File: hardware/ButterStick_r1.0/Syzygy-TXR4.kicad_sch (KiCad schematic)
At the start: 19 parts, among them J5 SYZYGY-TXR-4, U15 TLV62569DRL

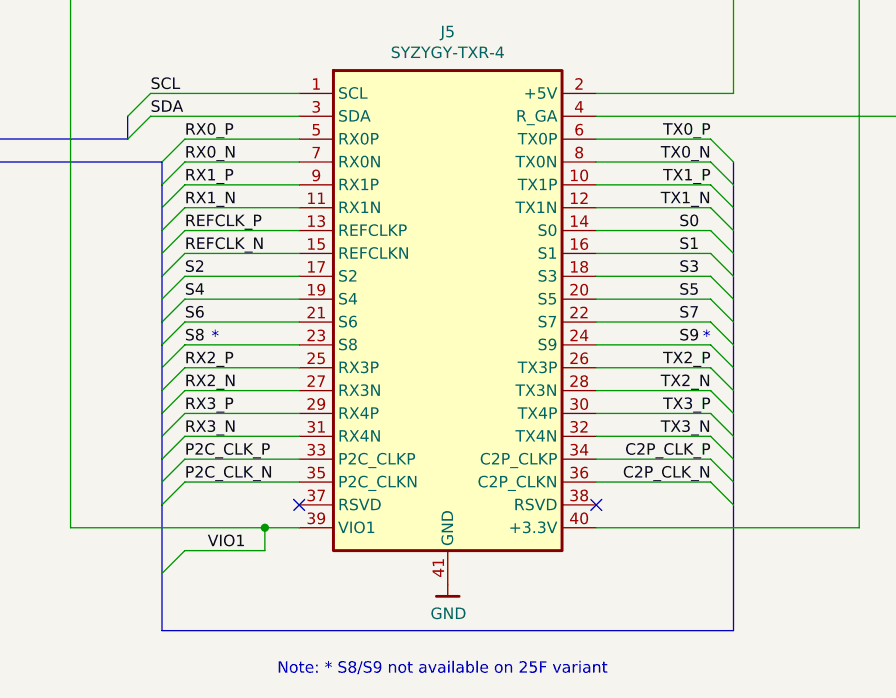
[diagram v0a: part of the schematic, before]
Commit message: hw.r1d0: Review complete, gerbers generated
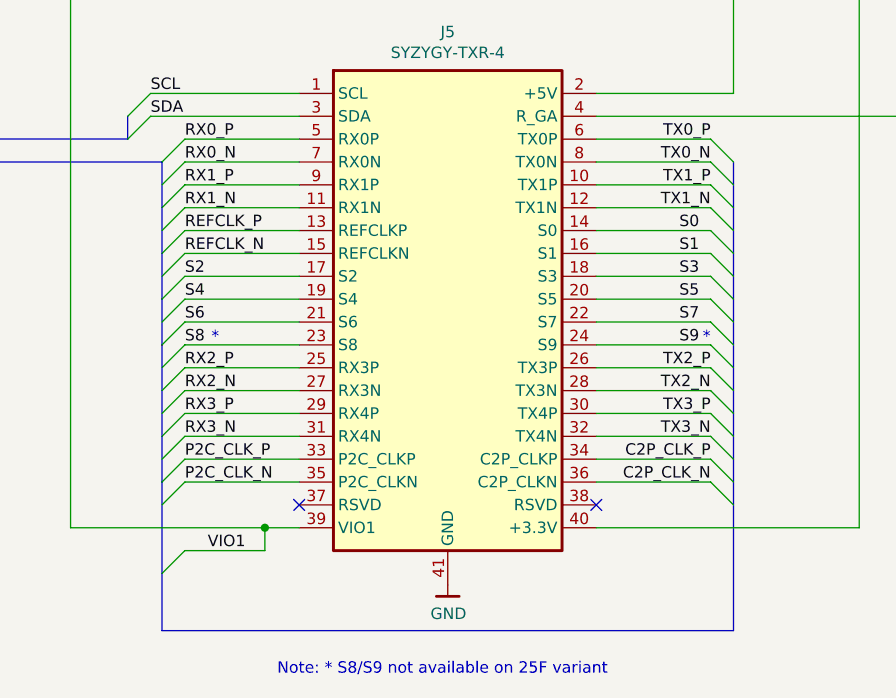
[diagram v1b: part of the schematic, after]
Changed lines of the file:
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@@
   (title_block
     (title "ButterStick")
-    (date "2020-07-16")
+    (date "2020-07-17")
     (rev "r1.0")
     (company "GsD")
@@
   (junction (at 137.16 39.37) (diameter 0) (color 0 0 0 0))
   (junction (at 176.53 142.24) (diameter 0) (color 0 0 0 0))
+  (no_connect (at 180.34 139.7))
   (no_connect (at 213.36 139.7))
-  (no_connect (at 180.34 139.7))
   (bus_entry (at 161.29 96.52) (size 2.54 -2.54)
     (stroke (width 0.1524) (type solid) (color 0 0 0 0))
@@
     (stroke (width 0) (type solid) (color 0 0 0 0))
   )
-  (bus (pts (xy 165.1 101.6) (xy 165.1 104.14))
-    (stroke (width 0) (type solid) (color 0 0 0 0))
-  )
-  (bus (pts (xy 165.1 104.14) (xy 165.1 109.22))
-    (stroke (width 0) (type solid) (color 0 0 0 0))
-  )
-  (bus (pts (xy 165.1 109.22) (xy 165.1 114.3))
-    (stroke (width 0) (type solid) (color 0 0 0 0))
-  )
-  (bus (pts (xy 165.1 114.3) (xy 165.1 119.38))
-    (stroke (width 0) (type solid) (color 0 0 0 0))
-  )
-  (bus (pts (xy 165.1 119.38) (xy 165.1 121.92))
+  (bus (pts (xy 165.1 101.6) (xy 165.1 106.68))
+    (stroke (width 0) (type solid) (color 0 0 0 0))
+  )
+  (bus (pts (xy 165.1 106.68) (xy 165.1 111.76))
+    (stroke (width 0) (type solid) (color 0 0 0 0))
+  )
+  (bus (pts (xy 165.1 111.76) (xy 165.1 116.84))
+    (stroke (width 0) (type solid) (color 0 0 0 0))
+  )
+  (bus (pts (xy 165.1 116.84) (xy 165.1 121.92))
     (stroke (width 0) (type solid) (color 0 0 0 0))
   )
@@
     (stroke (width 0) (type solid) (color 0 0 0 0))
   )
-  (bus (pts (xy 165.1 127) (xy 165.1 129.54))
-    (stroke (width 0) (type solid) (color 0 0 0 0))
-  )
-  (bus (pts (xy 165.1 129.54) (xy 165.1 134.62))
-    (stroke (width 0) (type solid) (color 0 0 0 0))
-  )
-  (bus (pts (xy 165.1 134.62) (xy 165.1 139.7))
-    (stroke (width 0) (type solid) (color 0 0 0 0))
-  )
-  (bus (pts (xy 165.1 139.7) (xy 165.1 153.67))
+  (bus (pts (xy 165.1 127) (xy 165.1 132.08))
+    (stroke (width 0) (type solid) (color 0 0 0 0))
+  )
+  (bus (pts (xy 165.1 132.08) (xy 165.1 137.16))
+    (stroke (width 0) (type solid) (color 0 0 0 0))
+  )
+  (bus (pts (xy 165.1 137.16) (xy 165.1 147.32))
+    (stroke (width 0) (type solid) (color 0 0 0 0))
+  )
+  (bus (pts (xy 165.1 147.32) (xy 165.1 153.67))
     (stroke (width 0) (type solid) (color 0 0 0 0))
   )
@@
     (stroke (width 0) (type solid) (color 0 0 0 0))
   )
-  (bus (pts (xy 228.6 127) (xy 228.6 132.08))
-    (stroke (width 0) (type solid) (color 0 0 0 0))
-  )
-  (bus (pts (xy 228.6 132.08) (xy 228.6 137.16))
-    (stroke (width 0) (type solid) (color 0 0 0 0))
-  )
+  (bus (pts (xy 228.6 127) (xy 228.6 129.54))
+    (stroke (width 0) (type solid) (color 0 0 0 0))
+  )
+  (bus (pts (xy 228.6 129.54) (xy 228.6 134.62))
+    (stroke (width 0) (type solid) (color 0 0 0 0))
+  )
+  (bus (pts (xy 228.6 134.62) (xy 228.6 137.16))
+    (stroke (width 0) (type solid) (color 0 0 0 0))
+  )
